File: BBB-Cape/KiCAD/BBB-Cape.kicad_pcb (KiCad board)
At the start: 2 copper layers, 75.3 x 54.6 mm, 60 parts, among them J1 01x06_Stackable Header, J2 RJ45-TRANSFO, P8 02x23_Stackable Header, P9 02x23_Stackable Header, SW1 W5500_RST, SW2 SYS_RST, SW3 Power, U1 WIZnet W5500, Y1 25MHz

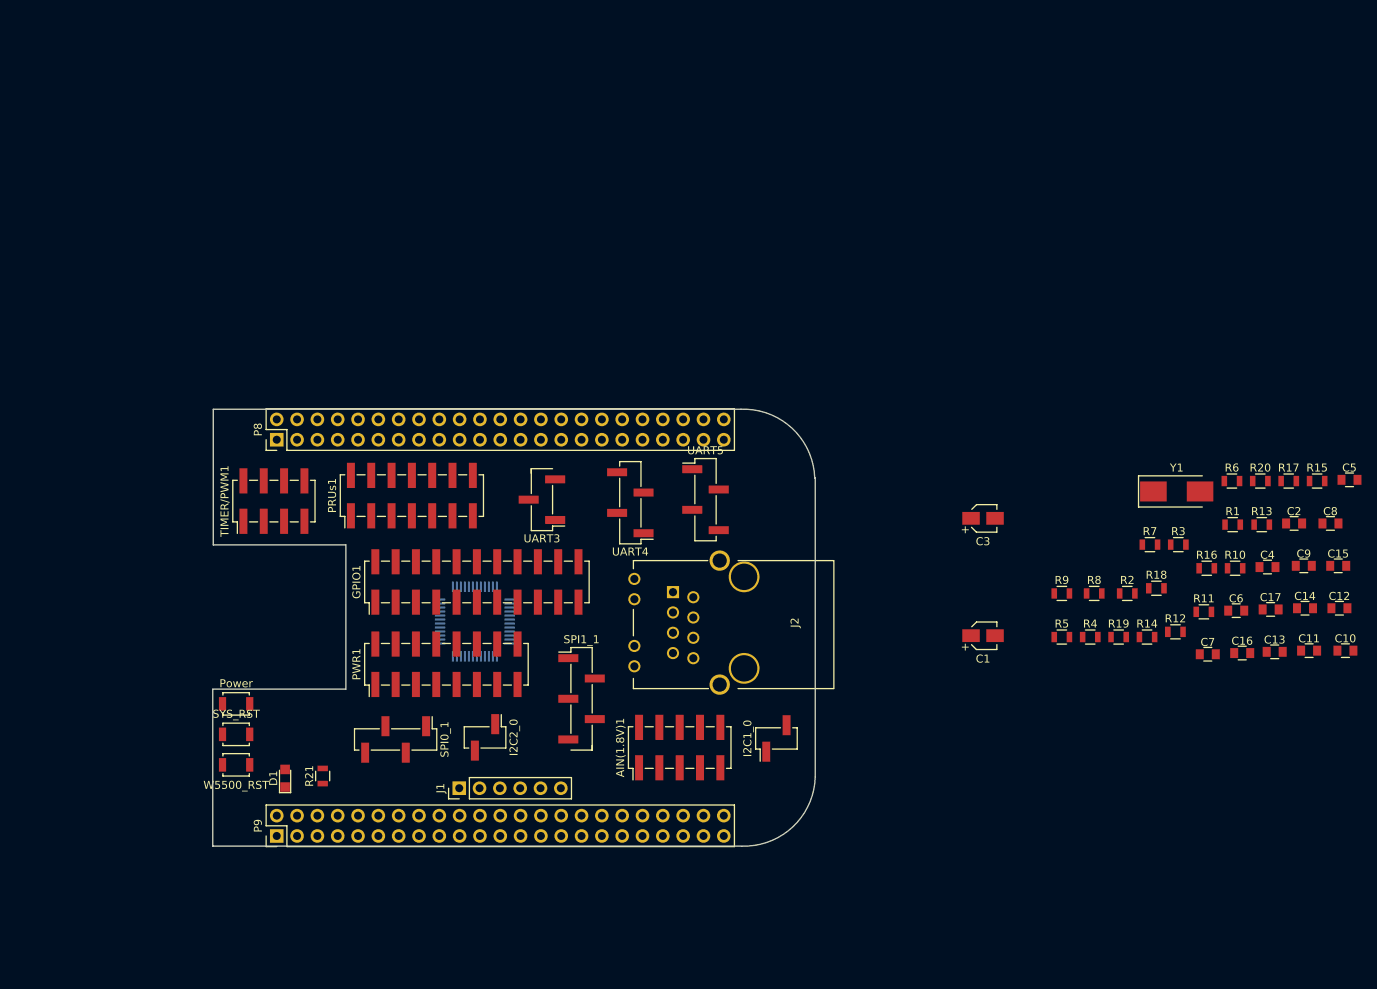
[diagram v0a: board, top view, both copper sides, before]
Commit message: BBB for review
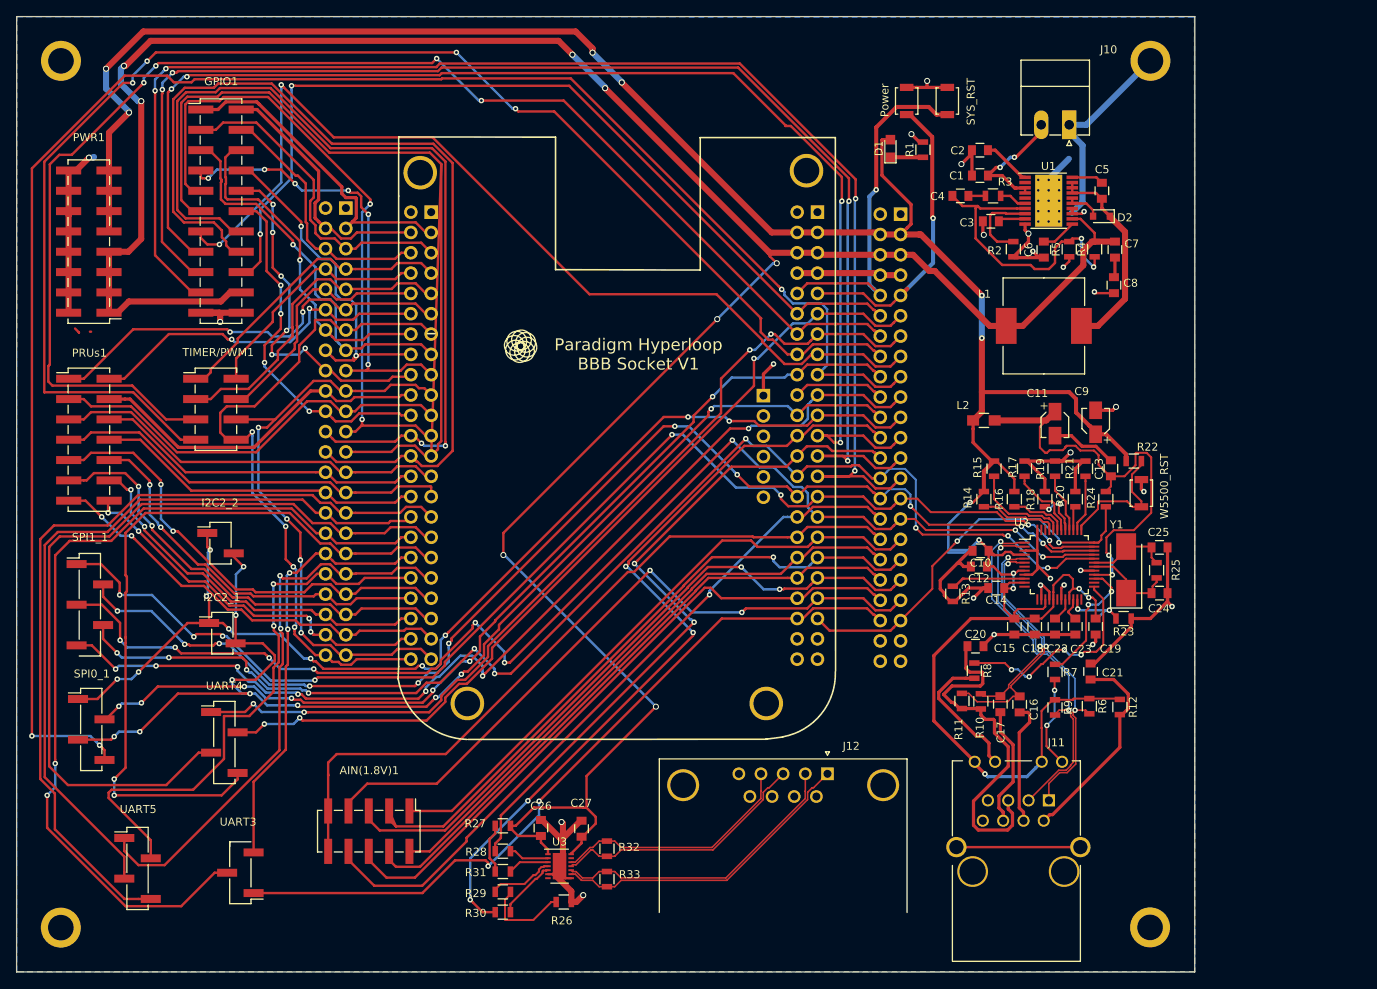
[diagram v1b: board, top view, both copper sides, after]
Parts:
- removed I2C1_0, I2C2_0: Conn_01x02, Pin_Headers:Pin_Header_Straight_1x02_Pitch2.54mm_SMD_Pin1Left
- removed P8, P9: 02x23_Stackable Header, Pin_Headers:Pin_Header_Straight_2x23_Pitch2.54mm
- added C18: 0.1uF, Capacitors_SMD:C_0805, F.Cu at (198.9, 99.6)
- added C19: 0.1uF, Capacitors_SMD:C_0805, F.Cu at (206.5, 99.6)
- added C20: 10nF, Capacitors_SMD:C_0805, F.Cu at (191.5, 102.0)
- added C21: 22nF, Capacitors_SMD:C_0805, F.Cu at (205.9, 105.2)
- added C22: 4.7uF, Capacitors_SMD:C_0805, F.Cu at (201.4, 99.6)
- added C23: 10nF, Capacitors_SMD:C_0805, F.Cu at (204.0, 99.6)
- added C24: 18pF, Capacitors_SMD:C_0805, F.Cu at (214.5, 95.4)
- added C25: 18pF, Capacitors_SMD:C_0805, F.Cu at (214.5, 89.7)
- added C26: 0.1uF, Capacitors_SMD:C_0805, F.Cu at (137.2, 124.7)
- added C27: 0.1uF, Capacitors_SMD:C_0805, F.Cu at (142.2, 124.8)
- added D2: 0.455V 20.0A, Diodes_SMD:D_0805, F.Cu at (207.2, 48.3)
- added I2C2_1: Conn_01x02, Pin_Headers:Pin_Header_Straight_1x02_Pitch2.54mm_SMD_Pin1Left, F.Cu at (97.3, 100.4)
- added I2C2_2: Conn_01x02, Pin_Headers:Pin_Header_Straight_1x02_Pitch2.54mm_SMD_Pin1Left, F.Cu at (97.1, 89.1)
- added J10: Conn_01x02, Connectors_Phoenix:PhoenixContact_MC-G_02x3.50mm_Angled, F.Cu at (203.2, 36.8)
- added J11: RJ45-TRANSFO, Connectors:RJ45_TRANSFO, F.Cu at (200.7, 121.3)
- added J12: DB9_Female, Connectors_DSub:DSUB-9_Female_Horizontal_Pitch2.77x2.84mm_EdgePinOffset14.56mm_Housed_MountingHolesOffset15.98mm, F.Cu at (173.0, 118.0)
- added J3: MOUNTING_HOLE, Mounting_Holes:MountingHole_3.2mm_M3_Pad, F.Cu at (122.1, 42.8)
- added J4: MOUNTING_HOLE, Mounting_Holes:MountingHole_3.2mm_M3_Pad, F.Cu at (170.4, 42.6)
- added J5: MOUNTING_HOLE, Mounting_Holes:MountingHole_3.2mm_M3_Pad, F.Cu at (213.3, 137.2)
- added J6: MOUNTING_HOLE, Mounting_Holes:MountingHole_3.2mm_M3_Pad, F.Cu at (213.4, 28.8)
- added J7: MOUNTING_HOLE, Mounting_Holes:MountingHole_3.2mm_M3_Pad, F.Cu at (77.1, 137.2)
- added J8: MOUNTING_HOLE, Mounting_Holes:MountingHole_3.2mm_M3_Pad, F.Cu at (77.2, 28.8)
- added J9: 01x06_Stackable Header, Pin_Headers:Pin_Header_Straight_1x06_Pitch2.54mm, B.Cu at (165.0, 70.7)
- added L1: 27.0uH, Inductors_SMD:L_Wuerth_HCM-1240, F.Cu at (200.0, 62.0)
- added L2: BLM21PG121SN1D, Inductors_SMD:L_0805_HandSoldering, F.Cu at (192.5, 73.8)
- added P1: 02x23_Stackable Header, Pin_Headers:Pin_Header_Straight_2x23_Pitch2.54mm, B.Cu at (171.7, 47.8)
- added P2: 02x23_Stackable Header, Pin_Headers:Pin_Header_Straight_2x23_Pitch2.54mm, B.Cu at (123.4, 47.8)
- added P3: 02x23_Stackable Header, Pin_Headers:Pin_Header_Straight_2x23_Pitch2.54mm, B.Cu at (112.8, 47.2)
- added P4: 02x23_Stackable Header, Pin_Headers:Pin_Header_Straight_2x23_Pitch2.54mm, B.Cu at (182.1, 48.0)
- added R22: 10k, Resistors_SMD:R_0805, F.Cu at (211.3, 78.9)
- added R23: 10k, Resistors_SMD:R_0805, F.Cu at (210.0, 98.6)
- added R24: 10k, Resistors_SMD:R_0805, F.Cu at (207.8, 83.6)
- added R25: 10M, Resistors_SMD:R_0805, F.Cu at (214.1, 92.5)
- added R26: 20k, Resistors_SMD:R_0805, F.Cu at (140.0, 134.0)
- added R27: 20k, Resistors_SMD:R_0805, F.Cu at (132.4, 124.5)
- added R28: 0, Resistors_SMD:R_0805, F.Cu at (132.4, 127.6)
- added R29: 0, Resistors_SMD:R_0805, F.Cu at (132.4, 132.7)
- added R30: 0, Resistors_SMD:R_0805, F.Cu at (132.4, 135.3)
- added R31: 0, Resistors_SMD:R_0805, F.Cu at (132.4, 130.2)
- added R32: 120, Resistors_SMD:R_0805, F.Cu at (145.4, 127.3)
- added R33: 120, Resistors_SMD:R_0805, F.Cu at (145.4, 131.1)
- added REF**: Paradigm Logo Very Small, Paradigm_Logo_Very_Small, F.Cu at (134.6, 64.5)
- added U2: WIZnet W5500, Housings_QFP:LQFP-48_7x7mm_Pitch0.5mm, F.Cu at (202.0, 91.8)
- added U3: MAX13433EETD, Housings_DFN_QFN:DFN-14-1EP_3x4mm_Pitch0.5mm, F.Cu at (139.5, 129.5)
- C1: value 10uF -> 1.00uF; footprint Capacitors_SMD:CP_Elec_3x5.3 -> Capacitors_SMD:C_0805
- C10: value 6.8nF -> 0.1uF
- C11: value 6.8nF -> 10uF; footprint Capacitors_SMD:C_0805 -> Capacitors_SMD:CP_Elec_3x5.3
- C12, C15: value 10nF -> 0.1uF
- C13: value 22nF -> 0.1uF
- C14: value 4.7uF -> 0.1uF
- C16, C17: value 18pF -> 6.8nF
- C3: value 10uF -> 270pF; footprint Capacitors_SMD:CP_Elec_3x5.3 -> Capacitors_SMD:C_0805
- C4: value 0.1uF -> 1.80nF
- C5: value 0.1uF -> 22nF
- C6: value 0.1uF -> 8.2nF
- C7, C8: value 0.1uF -> 47uF
- C9: value 0.1uF -> 10uF; footprint Capacitors_SMD:C_0805 -> Capacitors_SMD:CP_Elec_3x5.3
- J1: value 01x06_Stackable Header -> MOUNTING_HOLE; footprint Pin_Headers:Pin_Header_Straight_1x06_Pitch2.54mm -> Mounting_Holes:MountingHole_3.2mm_M3_Pad
- J2: value RJ45-TRANSFO -> MOUNTING_HOLE; footprint Connectors:RJ45_TRANSFO -> Mounting_Holes:MountingHole_3.2mm_M3_Pad
- R1: value 49.9 -> 330
- R10, R11: value 10k -> 82
- R12: value 10k -> 10
- R13: value 10k -> 12.4k
- R2: value 49.9 -> 16.2k
- R20: value 10M -> 10k
- R21: value 330 -> 10k
- R3: value 10 -> 22.1k
- R4: value 330 -> 3.09k
- R5: value 330 -> 1.02k
- R6: value 82 -> 49.9
- R7: value 82 -> 330
- R8: value 12.4k -> 330
- R9: value 10k -> 49.9
- U1: value WIZnet W5500 -> LM25576MH; footprint Housings_QFP:LQFP-48_7x7mm_Pitch0.5mm -> Housings_SSOP:HTSSOP-20-1EP_4.4x6.5mm_Pitch0.65mm_ThermalPad; moved to F.Cu
- moved SW2 119.0 mm to (188.0, 33.9), turned to 90 degrees
- moved SW1 118.1 mm to (212.2, 82.9), turned to 90 degrees
- moved SW3 112.7 mm to (182.9, 33.9), turned to 90 degrees
- moved D1 109.2 mm to (180.8, 39.8)
- moved R21 102.8 mm to (205.2, 79.8), turned to 270 degrees
- moved U1 88.9 mm to (200.6, 46.3)
- moved UART5 84.7 mm to (86.7, 129.8)
- moved PWR1 69.2 mm to (80.6, 51.4), turned to 180 degrees
- moved SPI1_1 62.6 mm to (80.8, 96.8)
- moved C2 61.0 mm to (192.0, 40.0), turned to 180 degrees
- moved R1 60.8 mm to (184.9, 39.9), turned to 90 degrees
- moved C4 60.2 mm to (189.6, 45.7)
- moved UART3 60.0 mm to (99.6, 130.3)
- moved UART4 58.9 mm to (97.6, 114.0), turned to 0 degrees
- moved C1 57.5 mm to (192.0, 43.2), turned to 180 degrees
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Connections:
- C1 pad 1: 3V3D -> Net-(C1-Pad1)
- C1 pad 2: Net-(C1-Pad2) -> DGND
- C10 pad 1: Net-(C10-Pad1) -> VDD_3V3
- C10 pad 2: RX+ -> DGND
- C11 pad 1: Net-(C11-Pad1) -> 3V3D
- C11 pad 2: RX- -> Net-(C11-Pad2)
- C12 pad 1: Net-(C12-Pad1) -> VDD_3V3
- C13 pad 1: Net-(C13-Pad1) -> 3V3D
- C13 pad 2: DGND -> Net-(C11-Pad2)
- C14 pad 1: Net-(C14-Pad1) -> VDD_3V3
- C15 pad 1: Net-(C15-Pad1) -> VDD_3V3
- C16 pad 2: DGND -> RX+
- C17 pad 2: DGND -> RX-
- C2 pad 1: 3V3D -> Net-(C2-Pad1)
- C2 pad 2: Net-(C1-Pad2) -> DGND
- C3 pad 1: VDD_3V3 -> Net-(C3-Pad1)
- C4 pad 1: VDD_3V3 -> Net-(C4-Pad1)
- C4 pad 2: DGND -> Net-(C4-Pad2)
- C5 pad 1: VDD_3V3 -> Net-(C5-Pad1)
- C5 pad 2: DGND -> Net-(C5-Pad2)
- C6 pad 1: VDD_3V3 -> Net-(C6-Pad1)
- C7 pad 1: VDD_3V3 -> VDD_5V
- C7 pad 2: DGND -> Net-(C7-Pad2)
- C8 pad 1: VDD_3V3 -> Net-(C7-Pad2)
- J2 pad 1: TX+ -> DGND
- R1 pad 1: VDD_3V3 -> Net-(D1-Pad1)
- R1 pad 2: TX+ -> DGND
- R10 pad 1: VDD_3V3 -> RX-
- R10 pad 2: Net-(R10-Pad2) -> Net-(C20-Pad1)
- R11 pad 1: VDD_3V3 -> RX+
- R11 pad 2: Net-(R11-Pad2) -> Net-(C20-Pad1)
- R12 pad 2: Net-(R12-Pad2) -> Net-(C21-Pad1)
- R13 pad 1: DGND -> Net-(R13-Pad1)
- R13 pad 2: Net-(R13-Pad2) -> DGND
- R14 pad 1: DGND -> VDD_3V3
- R15 pad 1: DGND -> VDD_3V3
- R16 pad 1: DGND -> VDD_3V3
- R18 pad 1: VDD_3V3 -> DGND
- R18 pad 2: W5500_RST -> Net-(R18-Pad2)
- R19 pad 1: 3V3D -> DGND
- R19 pad 2: W5500_INT -> Net-(R19-Pad2)
- R2 pad 1: VDD_3V3 -> DGND
- R2 pad 2: TX- -> Net-(R2-Pad2)
- R20 pad 1: Net-(C16-Pad1) -> DGND
- R20 pad 2: Net-(C17-Pad1) -> Net-(R20-Pad2)
- R21 pad 1: Net-(D1-Pad1) -> DGND
- R21 pad 2: DGND -> Net-(R21-Pad2)
- R3 pad 1: VDD_3V3 -> Net-(R3-Pad1)
- R3 pad 2: Net-(C13-Pad1) -> Net-(C4-Pad2)
- R4 pad 1: ACT_LED -> Net-(C4-Pad1)
- R4 pad 2: Net-(J2-PadGK) -> VDD_5V
- R5 pad 1: LINK_LED -> DGND
- R5 pad 2: Net-(J2-PadYK) -> Net-(C4-Pad1)
- R6 pad 1: RX- -> VDD_3V3
- R6 pad 2: Net-(C12-Pad1) -> TX+
- R7 pad 1: RX+ -> ACT_LED
- R7 pad 2: Net-(C12-Pad1) -> Net-(J11-PadGK)
- R8 pad 1: Net-(R8-Pad1) -> LINK_LED
- R8 pad 2: DGND -> Net-(J11-PadYK)
- R9 pad 1: DGND -> VDD_3V3
- R9 pad 2: Net-(R9-Pad2) -> TX-
- U1 pad 1: TX- -> Net-(C2-Pad1)
- U1 pad 10: Net-(R8-Pad1) -> DGND
- U1 pad 11: VDD_3V3 -> Net-(C6-Pad1)
- U1 pad 12: Net-(U1-Pad12) -> VDD_5V
- U1 pad 13: Net-(U1-Pad13) -> DGND
- U1 pad 15: VDD_3V3 -> Net-(D2-Pad2)
- U1 pad 16: DGND -> Net-(D2-Pad2)
- U1 pad 17: VDD_3V3 -> Net-(C5-Pad1)
- U1 pad 18: Net-(U1-Pad18) -> Net-(C5-Pad1)
- U1 pad 19: DGND -> Net-(C5-Pad1)
- U1 pad 2: TX+ -> Net-(U1-Pad2)
- U1 pad 20: Net-(C14-Pad1) -> Net-(C5-Pad2)
- U1 pad 21: VDD_3V3 -> (no net)
- U1 pad 3: DGND -> Net-(C1-Pad1)
- U1 pad 4: VDD_3V3 -> Net-(C1-Pad1)
- U1 pad 5: RX- -> Net-(U1-Pad5)
- U1 pad 6: RX+ -> Net-(R3-Pad1)
- U1 pad 7: Net-(U1-Pad7) -> Net-(C4-Pad1)
- U1 pad 8: VDD_3V3 -> Net-(R2-Pad2)
- U1 pad 9: DGND -> Net-(C3-Pad1)
- Y1 pad 1: Net-(C16-Pad1) -> Net-(C24-Pad1)
- Y1 pad 2: Net-(C17-Pad1) -> Net-(C25-Pad1)
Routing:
- net VDD_3V3: track 0.00 -> 342.2 mm, vias 0 -> 13
- net VDD_5V: track 0.00 -> 324.9 mm, vias 0 -> 8
- net DGND: track 0.00 -> 222.5 mm, vias 0 -> 25
- net I2C1_SCL/SPI0_CS0: track 0.00 -> 219.1 mm, vias 0 -> 3
- net EHRPWM1B: track 0.00 -> 178.7 mm, vias 0 -> 4
- net GPIO_115: track 0.00 -> 177.0 mm, vias 0 -> 4
- net EHRPWM1A: track 0.00 -> 172.7 mm, vias 0 -> 4
- net GPIO_117: track 0.00 -> 169.6 mm, vias 0 -> 4
- net GPIO49: track 0.00 -> 160.9 mm, vias 0 -> 4
- net SPI1_CS0: track 0.00 -> 157.9 mm, vias 0 -> 10
- net SPI1_SCLK: track 0.00 -> 157.7 mm, vias 0 -> 9
- net SPI1_D0: track 0.00 -> 155.9 mm, vias 0 -> 8
- net SPI1_DI: track 0.00 -> 154.6 mm, vias 0 -> 11
- net I2C2_SDA/SPIO_SCLK/UART2_RXD: track 0.00 -> 149.9 mm, vias 0 -> 10
- net I2C2_SCL/SPI0_DO/UART2_TXD: track 0.00 -> 138.1 mm, vias 0 -> 10
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- added copper zone on B.Cu, net DGND
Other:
- board size 75.3 x 54.6 mm -> 147.3 x 119.4 mm
- net class Default: clearance 0.254 -> 0.2; trace_width 0.254 -> 0.4064
- net class Signal added: clearance 0.1, trace_width 0.2, via_dia 0.6858, via_drill 0.3302
- net class VCC added: clearance 0.254, trace_width 0.508, via_dia 0.6858, via_drill 0.3302
- rule trace_clearance: 0.254 -> 0.2
- board text added: "Paradigm Hyperloop BBB Socket V1"
